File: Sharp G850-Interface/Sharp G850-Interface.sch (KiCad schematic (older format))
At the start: 28 parts, among them J1 USB_B_Micro, J2 Conn_01x11_Male, J3 Conn_01x11_Male, U1 FT232RL

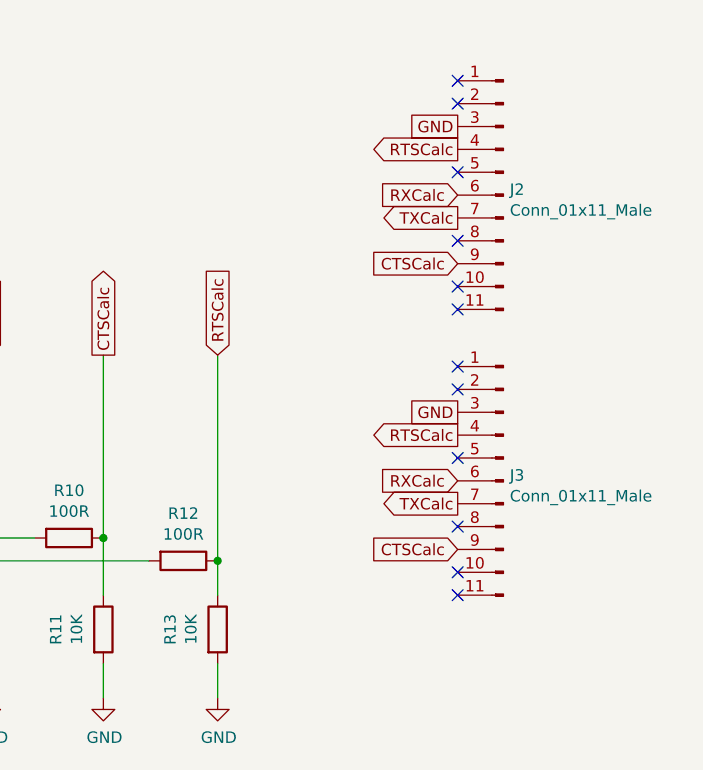
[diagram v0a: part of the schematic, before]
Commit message: Finished PCB + Added gerber files
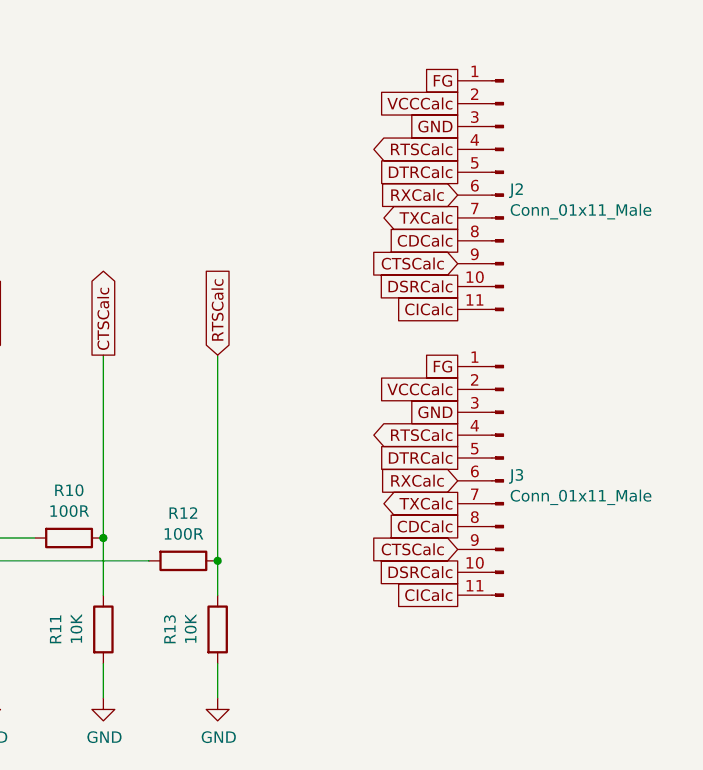
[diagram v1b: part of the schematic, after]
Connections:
- net FG: now reaches J2.1 (Pin_1)
- net FG: now also J3.1 (Pin_1)
- net DSRCalc: now reaches J2.10 (Pin_10)
- net DSRCalc: now also J3.10 (Pin_10)
- net CICalc: now reaches J2.11 (Pin_11)
- net CICalc: now also J3.11 (Pin_11)
- net VCCCalc: now reaches J2.2 (Pin_2)
- net VCCCalc: now also J3.2 (Pin_2)
- net DTRCalc: now reaches J2.5 (Pin_5)
- net DTRCalc: now also J3.5 (Pin_5)
- net CDCalc: now reaches J2.8 (Pin_8)
- net CDCalc: now also J3.8 (Pin_8)
- no-connect marks 22 -> 10
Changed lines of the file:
@@
 Text GLabel 10050 1800 0    50   Input ~ 0
 CTSCalc
-NoConn ~ 10050 1400
-NoConn ~ 10050 1700
-NoConn ~ 10050 1900
 $Comp
 L Device:R R6
@@
 	1    0    0    -1
 $EndComp
-NoConn ~ 10050 1100
 Wire Wire Line
 	5200 3500 4850 3500
@@
 	1    0    0    -1
 $EndComp
-NoConn ~ 10050 1000
 $Comp
 L Connector:Conn_01x11_Male J2
@@
 	-1   0    0    -1
 $EndComp
-NoConn ~ 10050 2000
 Wire Wire Line
 	3800 1650 3750 1650
@@
 Text GLabel 10050 3050 0    50   Input ~ 0
 CTSCalc
-NoConn ~ 10050 2650
-NoConn ~ 10050 2950
-NoConn ~ 10050 3150
-NoConn ~ 10050 2350
-NoConn ~ 10050 2250
-$Comp
-L Connector:Conn_01x11_Male J3
-U 1 1 5EC5BD70
-P 10250 2750
-F 0 "J3" H 10222 2774 50  0000 R CNN
-F 1 "Conn_01x11_Male" H 10222 2683 50  0000 R CNN
-F 2 "Connector_PinHeader_2.54mm:PinHeader_1x11_P2.54mm_Vertical" H 10250 2750 50  0001 C CNN
-F 3 "~" H 10250 2750 50  0001 C CNN
-	1    10250 2750
-	-1   0    0    -1
-$EndComp
-NoConn ~ 10050 3250
 $Comp
 L Device:Ferrite_Bead_Small FB1
@@
 Text Label 4150 3200 0    50   ~ 0
 USBD-
+$Comp
+L Connector:Conn_01x11_Male J3
+U 1 1 5EC5BD70
+P 10250 2750
+F 0 "J3" H 10222 2774 50  0000 R CNN
+F 1 "Conn_01x11_Male" H 10222 2683 50  0000 R CNN
+F 2 "Connector_PinHeader_2.54mm:PinHeader_1x11_P2.54mm_Vertical" H 10250 2750 50  0001 C CNN
+F 3 "~" H 10250 2750 50  0001 C CNN
+	1    10250 2750
+	-1   0    0    -1
+$EndComp
+Text GLabel 10050 1000 0    50   UnSpc ~ 0
+FG
+Text GLabel 10050 1100 0    50   UnSpc ~ 0
+VCCCalc
+Text GLabel 10050 1400 0    50   UnSpc ~ 0
+DTRCalc
+Text GLabel 10050 1700 0    50   UnSpc ~ 0
+CDCalc
+Text GLabel 10050 1900 0    50   UnSpc ~ 0
+DSRCalc
+Text GLabel 10050 2000 0    50   UnSpc ~ 0
+CICalc
+Text GLabel 10050 2250 0    50   UnSpc ~ 0
+FG
+Text GLabel 10050 2350 0    50   UnSpc ~ 0
+VCCCalc
+Text GLabel 10050 2650 0    50   UnSpc ~ 0
+DTRCalc
+Text GLabel 10050 2950 0    50   UnSpc ~ 0
+CDCalc
+Text GLabel 10050 3150 0    50   UnSpc ~ 0
+DSRCalc
+Text GLabel 10050 3250 0    50   UnSpc ~ 0
+CICalc
 $EndSCHEMATC
